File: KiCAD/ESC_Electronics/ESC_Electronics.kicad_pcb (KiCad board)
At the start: 2 copper layers, 64 parts, among them J1 -1000VDC, J2 Test Input, J3 CA probe, J4 DC Power, J5 Output, J6 Barrel_Jack, J7 -6V, J8 +6V, Q1 MMBT3906, Q2 MMBT3904, U1 CR110, U2 SiPhotodiode, U3 TL072, U4 LM317, U5 TLE2426xP

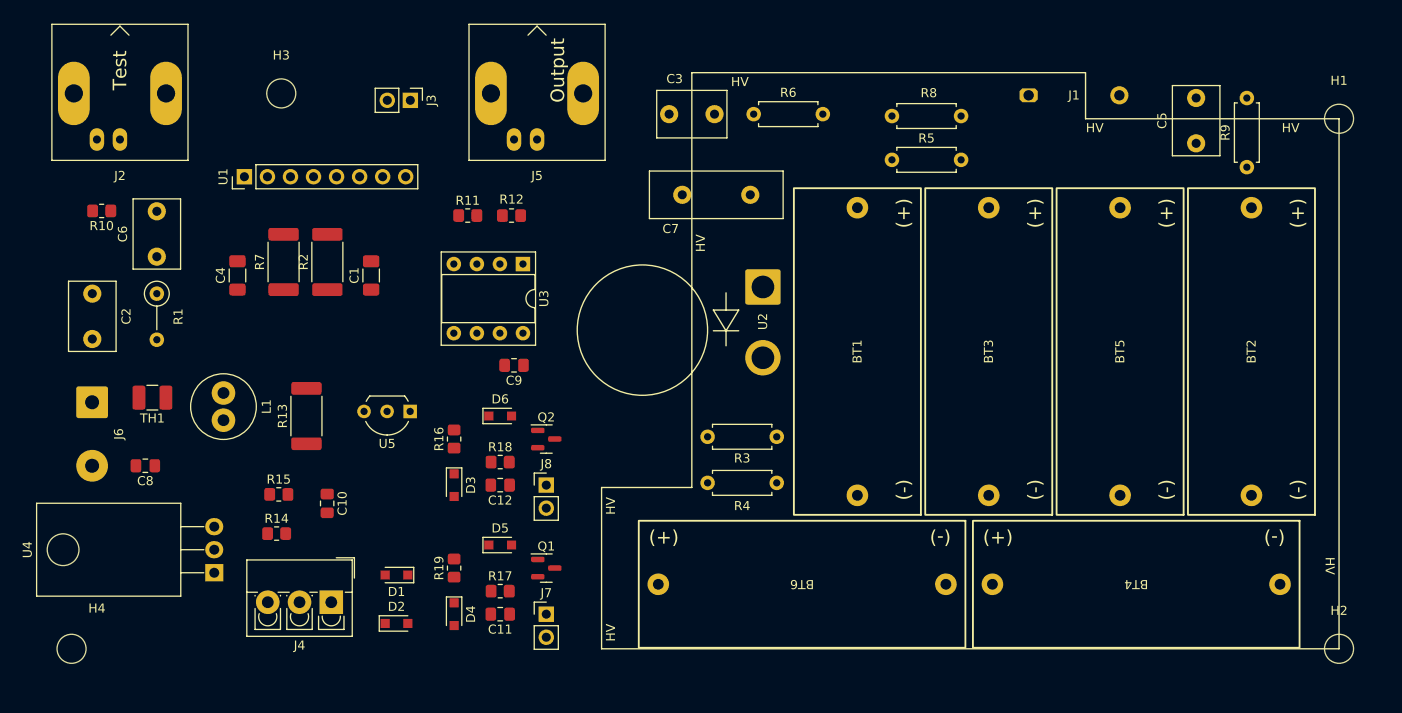
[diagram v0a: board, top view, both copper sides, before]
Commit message: layed out board
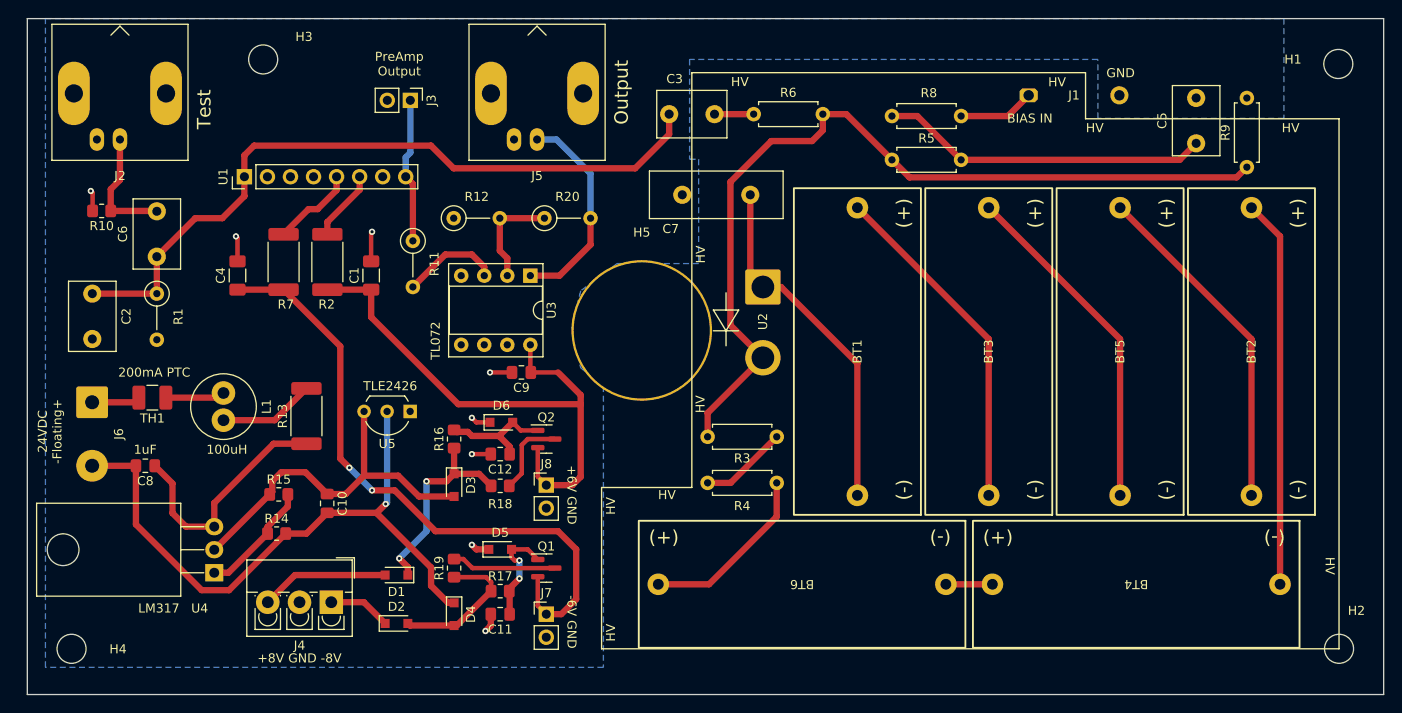
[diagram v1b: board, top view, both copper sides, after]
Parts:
- added H5: DiodeFeedThru, ESC_Electronics_Library:DiodeFeedThru, F.Cu at (118.7, 89.4)
- added R20: 10k, Resistor_THT:R_Axial_DIN0207_L6.3mm_D2.5mm_P5.08mm_Vertical, F.Cu at (108.0, 77.0)
- C6: value 1nF -> 1pF
- R11: footprint Resistor_SMD:R_0805_2012Metric_Pad1.20x1.40mm_HandSolder -> Resistor_THT:R_Axial_DIN0207_L6.3mm_D2.5mm_P5.08mm_Vertical
- R12: value 20k -> 10k; footprint Resistor_SMD:R_0805_2012Metric_Pad1.20x1.40mm_HandSolder -> Resistor_THT:R_Axial_DIN0207_L6.3mm_D2.5mm_P5.08mm_Vertical
- moved R11 6.66 mm to (93.5, 79.5), turned to -90 degrees
- moved R12 6.38 mm to (98.0, 77.0), turned to 0 degrees
- moved H1 6.04 mm to (195.5, 60.0)
- moved H3 4.24 mm to (77.0, 59.5)
- moved C12 3.42 mm to (103.1, 103.0)
- moved R18 2.62 mm to (103.1, 106.5)
- moved U3 1.52 mm to (106.4, 83.3)
- moved C9 1.13 mm to (105.5, 94.0)
- moved D6 0.71 mm to (103.2, 99.5)
- moved D5 0.47 mm to (103.1, 113.5)
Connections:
- C9 pad 2: Net-(C9-Pad2) -> GND
- R12 pad 1: Net-(J5-Pad1) -> GND
- R12 pad 2: Net-(R11-Pad2) -> Net-(R12-Pad2)
- U3 pad 2: Net-(C9-Pad2) -> Net-(R12-Pad2)
- U3 pad 4: Net-(C9-Pad2) -> GND
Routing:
- net Net-(R3-Pad2): track 0.00 -> 96.5 mm
- net Net-(C2-Pad1): track 0.00 -> 80.2 mm
- net -6VDC: track 0.00 -> 70.4 mm, vias 0 -> 2
- net Net-(C10-Pad2): track 0.00 -> 69.9 mm, vias 0 -> 1
- net +6VDC: track 0.00 -> 62.2 mm
- net Net-(BT2-Pad1): track 0.00 -> 42.8 mm
- net Net-(C10-Pad1): track 0.00 -> 40.5 mm
- net Net-(BT1-Pad2): track 0.00 -> 39.2 mm
- net Net-(BT2-Pad2): track 0.00 -> 37.7 mm
- net Net-(BT1-Pad1): track 0.00 -> 37.7 mm
- net Net-(BT3-Pad1): track 0.00 -> 37.7 mm
- net Net-(C5-Pad1): track 0.00 -> 36.3 mm
- net Net-(C8-Pad1): track 0.00 -> 26.7 mm
- net Net-(J5-Pad1): track 0.00 -> 23.3 mm
- net Net-(D1-Pad1): track 0.00 -> 22.8 mm, vias 0 -> 2
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- added copper zone on B.Cu, net GND
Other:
- board outline added: 149.5 x 74.5 mm
- board text added: "+6V GND"
- board text added: "+8V GND -8V"
- board text added: "-6V GND"
- board text added: "100uH"
- board text added: "1uF"
- board text added: "200mA PTC"
- board text added: "24VDC -Floating+"
- board text added: "BIAS IN"
- board text added: "GND"
- board text added: "LM317"
- board text added: "PreAmp Output"
- board text added: "TL072"
- board text added: "TLE2426"
